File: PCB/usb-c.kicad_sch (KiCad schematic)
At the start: 14 parts, among them J4 TYPE-C-31-M-12, U17 TPS62132, U3 TPD2EUSB30

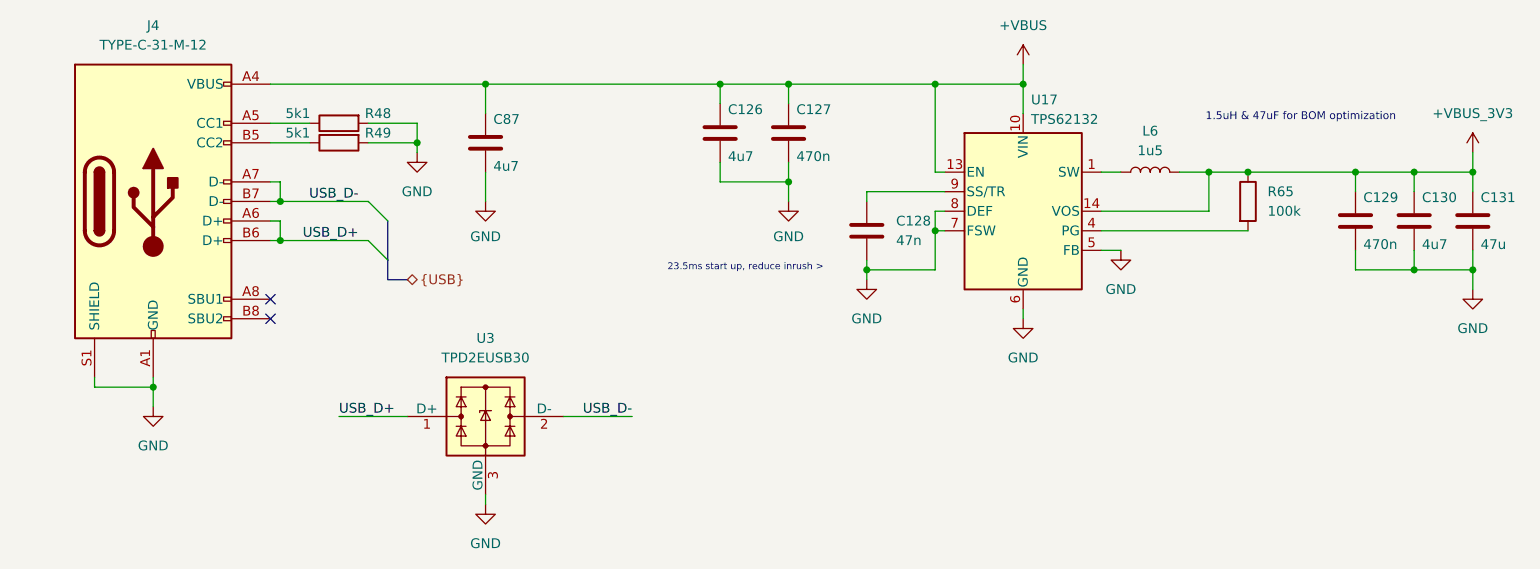
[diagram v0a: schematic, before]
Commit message: new power rail YAY
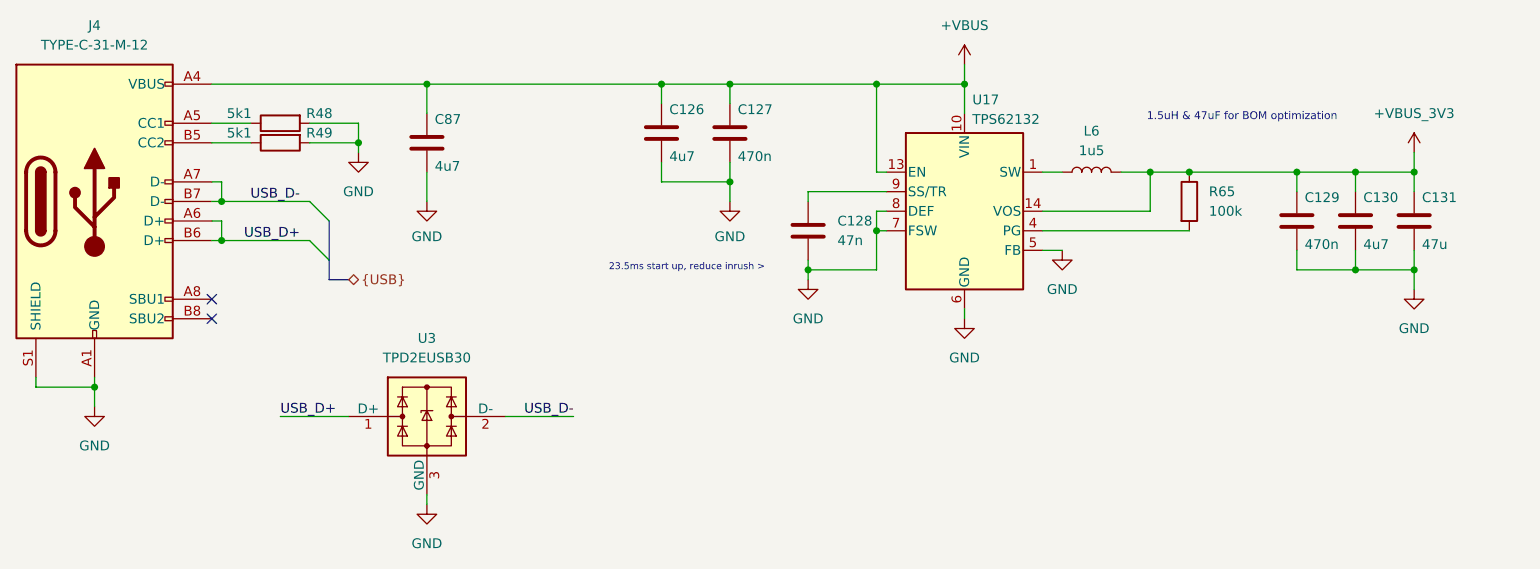
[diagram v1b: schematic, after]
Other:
- moved on the sheet: C126, C127, C128, C129, C130, C131, C87, J4, L6, R48, R49, R65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
